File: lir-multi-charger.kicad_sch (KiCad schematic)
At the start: 29 parts, among them J1 USB_C_Receptacle_USB2.0, J2 Conn_01x02_Male, U1 TP4056, U2 TP4056

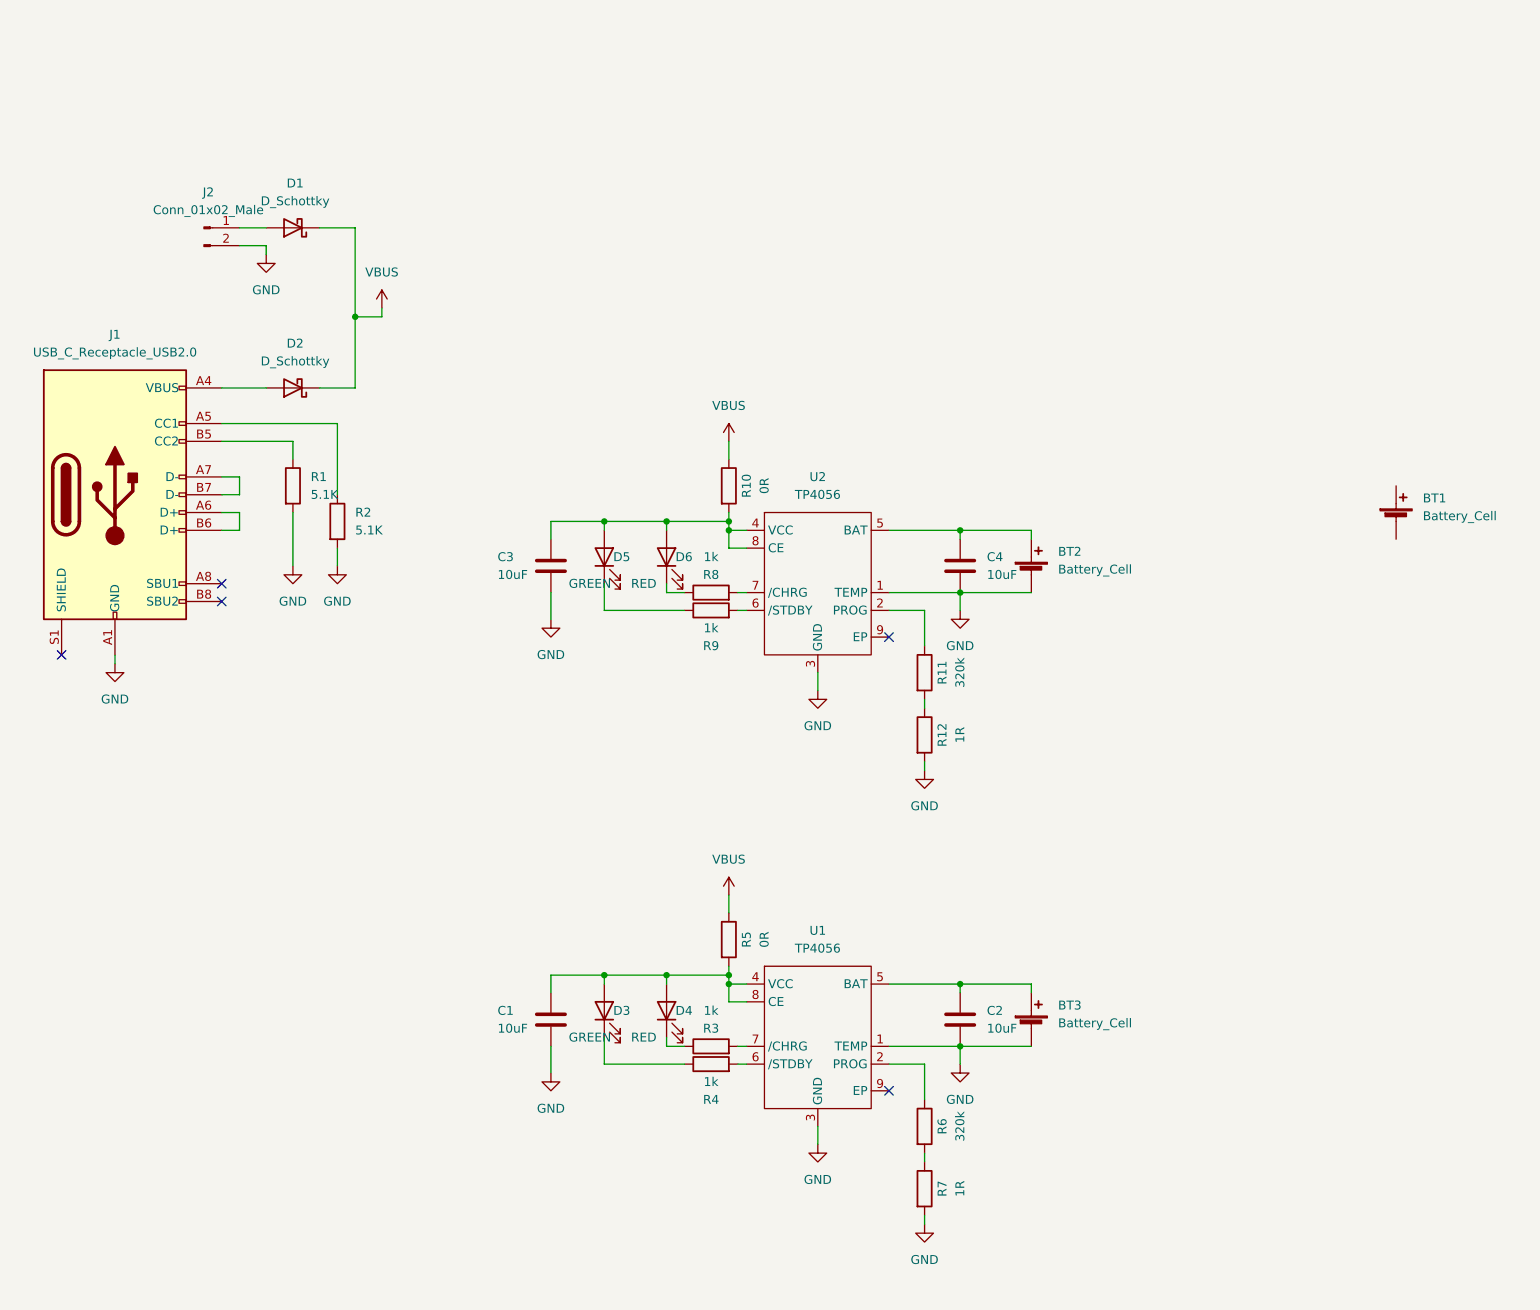
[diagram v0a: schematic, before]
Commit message: placing components
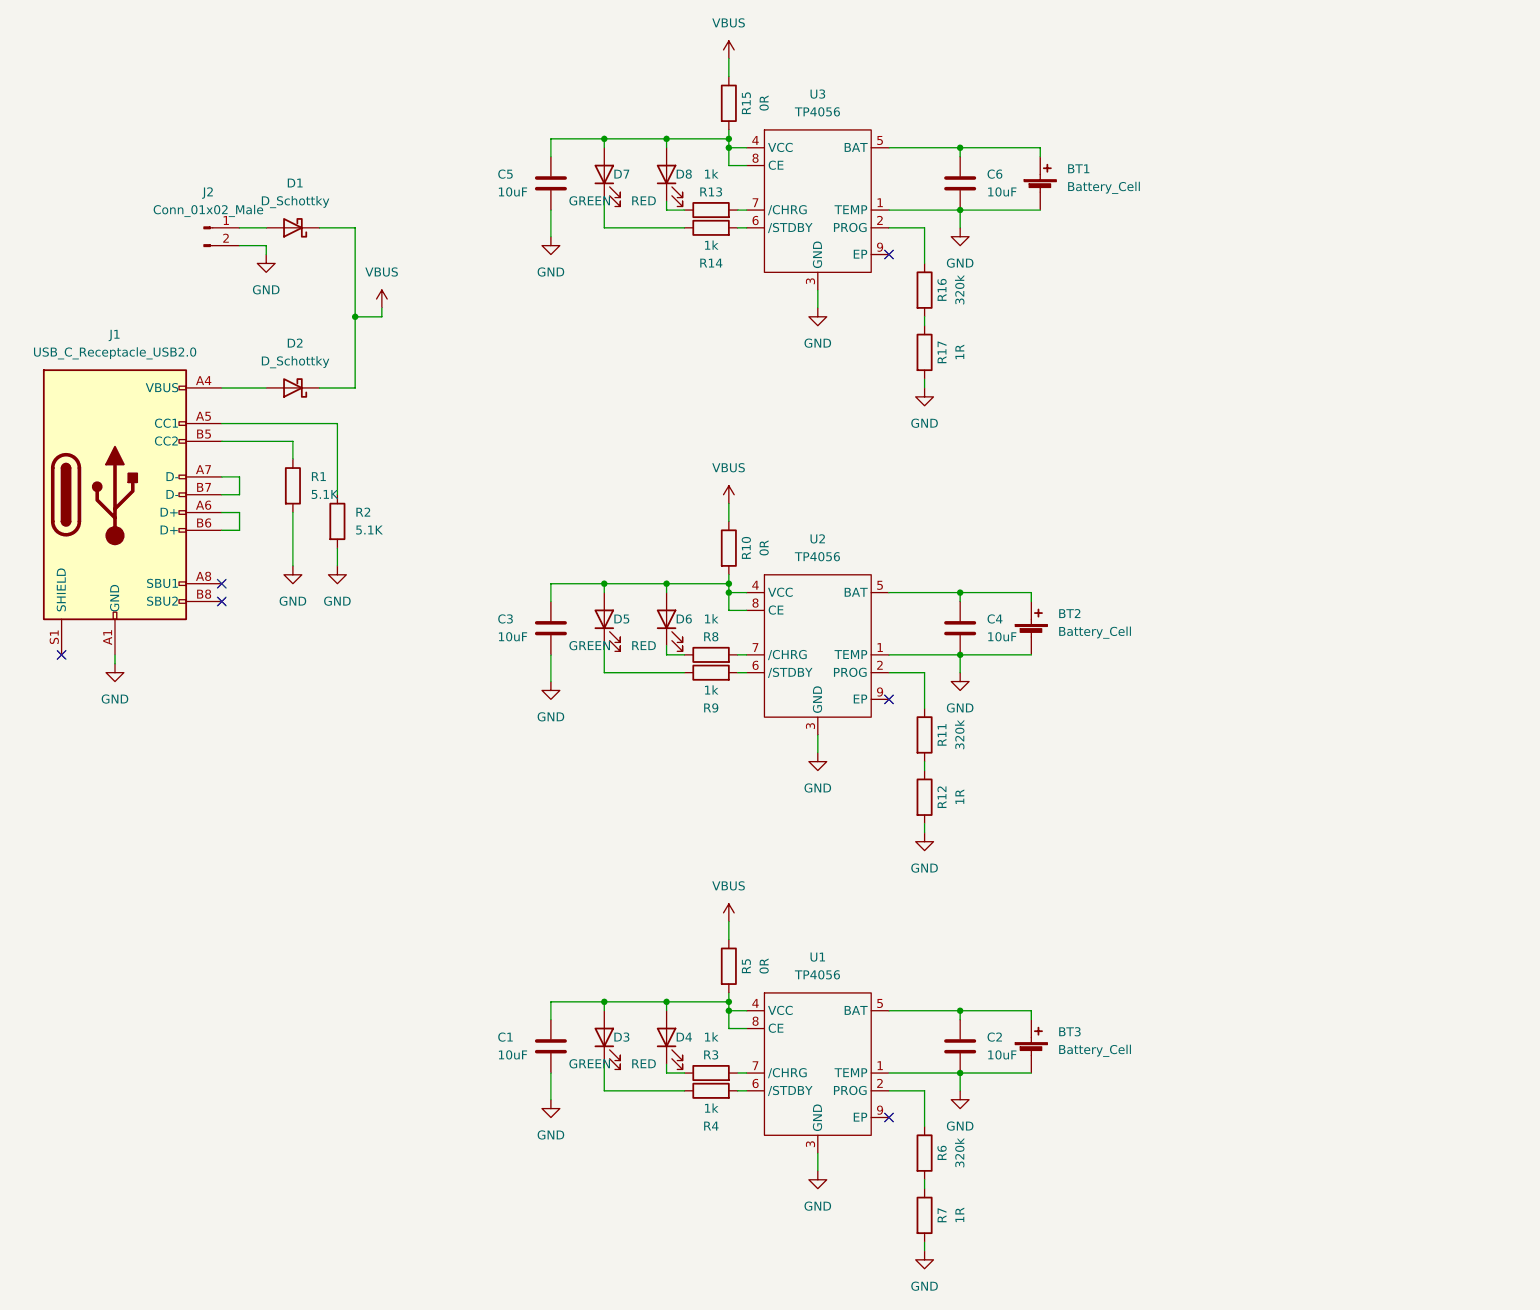
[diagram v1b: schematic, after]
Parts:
- added C5, C6: 10uF, Capacitor_SMD:C_0805_2012Metric_Pad1.18x1.45mm_HandSolder, symbol Device:C
- added D7: GREEN, LED_SMD:LED_0805_2012Metric_Pad1.15x1.40mm_HandSolder, symbol Device:LED
- added D8: RED, LED_SMD:LED_0805_2012Metric_Pad1.15x1.40mm_HandSolder, symbol Device:LED
- added R13, R14: 1k, Resistor_SMD:R_0805_2012Metric_Pad1.20x1.40mm_HandSolder, symbol Device:R
- added R15: 0R, Resistor_SMD:R_0805_2012Metric_Pad1.20x1.40mm_HandSolder, symbol Device:R
- added R16: 320k, Resistor_SMD:R_0805_2012Metric_Pad1.20x1.40mm_HandSolder, symbol Device:R
- added R17: 1R, Resistor_SMD:R_0805_2012Metric_Pad1.20x1.40mm_HandSolder, symbol Device:R
- added U3: TP4056, Li-ion-charger:tp4056, symbol Li_ion_charger:TP4056
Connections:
- net GND: now also BT1.2 (-), C5.2, C6.2, R17.2, U3.1 (TEMP), U3.3 (GND)
- net VBUS: now also R15.1
- net at BT1.1 (+): now also C6.1, U3.5 (BAT)
- new net: R16.1, U3.2 (PROG)
- new net: C5.1, D7.2 (A), D8.2 (A), R15.2, U3.4 (VCC), U3.8 (CE)
- new net: R14.2, U3.6 (/STDBY)
- new net: R13.2, U3.7 (/CHRG)
- new net: D8.1 (K), R13.1
- new net: D7.1 (K), R14.1
- new net: R16.2, R17.1
- no-connect marks 5 -> 6
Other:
- moved on the sheet: BT1, BT2, BT3, C1, C2, C3, C4, D3, D4, D5, D6, R10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
